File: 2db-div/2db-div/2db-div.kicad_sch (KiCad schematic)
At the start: 34 parts, among them J1001 Conn_01x02, J1002 From R2, J1003 Conn_01x02, J1004 Conn_Coaxial, SW1001 2dB, SW1002 Video, U1001 MC1458

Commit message: minor changes for spice
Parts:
- H1001, H1002, H1003, H1004, SW1002: Spice_Netlist_Enabled (none) -> N; Spice_Primitive (none) -> R
- J1002: Spice_Model (none) -> From R2; Spice_Netlist_Enabled (none) -> N; Spice_Primitive (none) -> J
- SW1001: Spice_Model (none) -> 2dB
- U1001: Spice_Lib_File 2db-div-spice\MC1458-dual.lib -> 2db-div-spice\LM358-dual.lib; Spice_Model MC1458_ti -> LM358c; Spice_Netlist_Enabled Y -> N
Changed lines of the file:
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@@
+      (effects (font (size 1.27 1.27)) hide)
+    )
+    (property "Spice_Primitive" "R" (id 4) (at 180.975 163.83 0)
+      (effects (font (size 1.27 1.27)) hide)
+    )
+    (property "Spice_Netlist_Enabled" "N" (id 5) (at 180.975 163.83 0)
       (effects (font (size 1.27 1.27)) hide)
     )
@@
       (effects (font (size 1.27 1.27)) hide)
     )
-    (property "Spice_Model" "MC1458_ti" (id 5) (at 132.08 82.55 0)
-      (effects (font (size 1.27 1.27)) hide)
-    )
-    (property "Spice_Netlist_Enabled" "Y" (id 6) (at 132.08 82.55 0)
-      (effects (font (size 1.27 1.27)) hide)
-    )
-    (property "Spice_Lib_File" "2db-div-spice\\MC1458-dual.lib" (id 7) (at 132.08 82.55 0)
+    (property "Spice_Model" "LM358c" (id 5) (at 132.08 82.55 0)
+      (effects (font (size 1.27 1.27)) hide)
+    )
+    (property "Spice_Netlist_Enabled" "N" (id 6) (at 132.08 82.55 0)
+      (effects (font (size 1.27 1.27)) hide)
+    )
+    (property "Spice_Lib_File" "2db-div-spice\\LM358-dual.lib" (id 7) (at 132.08 82.55 0)
       (effects (font (size 1.27 1.27)) hide)
     )
@@
       (effects (font (size 1.27 1.27)) hide)
     )
+    (property "Spice_Primitive" "R" (id 4) (at 227.33 85.09 0)
+      (effects (font (size 1.27 1.27)) hide)
+    )
+    (property "Spice_Netlist_Enabled" "N" (id 5) (at 227.33 85.09 0)
+      (effects (font (size 1.27 1.27)) hide)
+    )
     (pin "1")
     (pin "2")
@@
       (effects (font (size 1.27 1.27)) hide)
     )
+    (property "Spice_Primitive" "R" (id 4) (at 217.805 163.83 0)
+      (effects (font (size 1.27 1.27)) hide)
+    )
+    (property "Spice_Netlist_Enabled" "N" (id 5) (at 217.805 163.83 0)
+      (effects (font (size 1.27 1.27)) hide)
+    )
   )
   (symbol (lib_id "Mechanical:MountingHole") (at 163.195 163.83 0) (unit 1)
@@
     )
     (property "Datasheet" "~" (id 3) (at 163.195 163.83 0)
+      (effects (font (size 1.27 1.27)) hide)
+    )
+    (property "Spice_Primitive" "R" (id 4) (at 163.195 163.83 0)
+      (effects (font (size 1.27 1.27)) hide)
+    )
+    (property "Spice_Netlist_Enabled" "N" (id 5) (at 163.195 163.83 0)
       (effects (font (size 1.27 1.27)) hide)
     )
@@
     )
     (property "Datasheet" "~" (id 3) (at 198.755 163.83 0)
+      (effects (font (size 1.27 1.27)) hide)
+    )
+    (property "Spice_Primitive" "R" (id 4) (at 198.755 163.83 0)
+      (effects (font (size 1.27 1.27)) hide)
+    )
+    (property "Spice_Netlist_Enabled" "N" (id 5) (at 198.755 163.83 0)
       (effects (font (size 1.27 1.27)) hide)
     )
@@
       (effects (font (size 1.27 1.27)) hide)
     )
+    (property "Spice_Model" "2dB" (id 6) (at 208.28 77.47 0)
+      (effects (font (size 1.27 1.27)) hide)
+    )
     (pin "1")
     (pin "2")
@@
       (effects (font (size 1.27 1.27)) hide)
     )
-    (property "Spice_Model" "MC1458_ti" (id 5) (at 155.575 80.01 0)
-      (effects (font (size 1.27 1.27)) hide)
-    )
-    (property "Spice_Netlist_Enabled" "Y" (id 6) (at 155.575 80.01 0)
-      (effects (font (size 1.27 1.27)) hide)
-    )
-    (property "Spice_Lib_File" "2db-div-spice\\MC1458-dual.lib" (id 7) (at 155.575 80.01 0)
+    (property "Spice_Model" "LM358c" (id 5) (at 155.575 80.01 0)
+      (effects (font (size 1.27 1.27)) hide)
+    )
+    (property "Spice_Netlist_Enabled" "N" (id 6) (at 155.575 80.01 0)
+      (effects (font (size 1.27 1.27)) hide)
+    )
+    (property "Spice_Lib_File" "2db-div-spice\\LM358-dual.lib" (id 7) (at 155.575 80.01 0)
       (effects (font (size 1.27 1.27)) hide)
     )
@@
       (effects (font (size 1.27 1.27)) hide)
     )
-    (property "Spice_Model" "MC1458_ti" (id 5) (at 158.75 80.01 0)
-      (effects (font (size 1.27 1.27)) hide)
-    )
-    (property "Spice_Netlist_Enabled" "Y" (id 6) (at 158.75 80.01 0)
-      (effects (font (size 1.27 1.27)) hide)
-    )
-    (property "Spice_Lib_File" "2db-div-spice\\MC1458-dual.lib" (id 7) (at 158.75 80.01 0)
+    (property "Spice_Model" "LM358c" (id 5) (at 158.75 80.01 0)
+      (effects (font (size 1.27 1.27)) hide)
+    )
+    (property "Spice_Netlist_Enabled" "N" (id 6) (at 158.75 80.01 0)
+      (effects (font (size 1.27 1.27)) hide)
+    )
+    (property "Spice_Lib_File" "2db-div-spice\\LM358-dual.lib" (id 7) (at 158.75 80.01 0)
       (effects (font (size 1.27 1.27)) hide)
     )
@@
       (effects (font (size 1.27 1.27)) hide)
     )
+    (property "Spice_Primitive" "J" (id 4) (at 72.39 85.09 0)
+      (effects (font (size 1.27 1.27)) hide)
+    )
+    (property "Spice_Model" "From R2" (id 5) (at 72.39 85.09 0)
+      (effects (font (size 1.27 1.27)) hide)
+    )
+    (property "Spice_Netlist_Enabled" "N" (id 6) (at 72.39 85.09 0)
+      (effects (font (size 1.27 1.27)) hide)
+    )

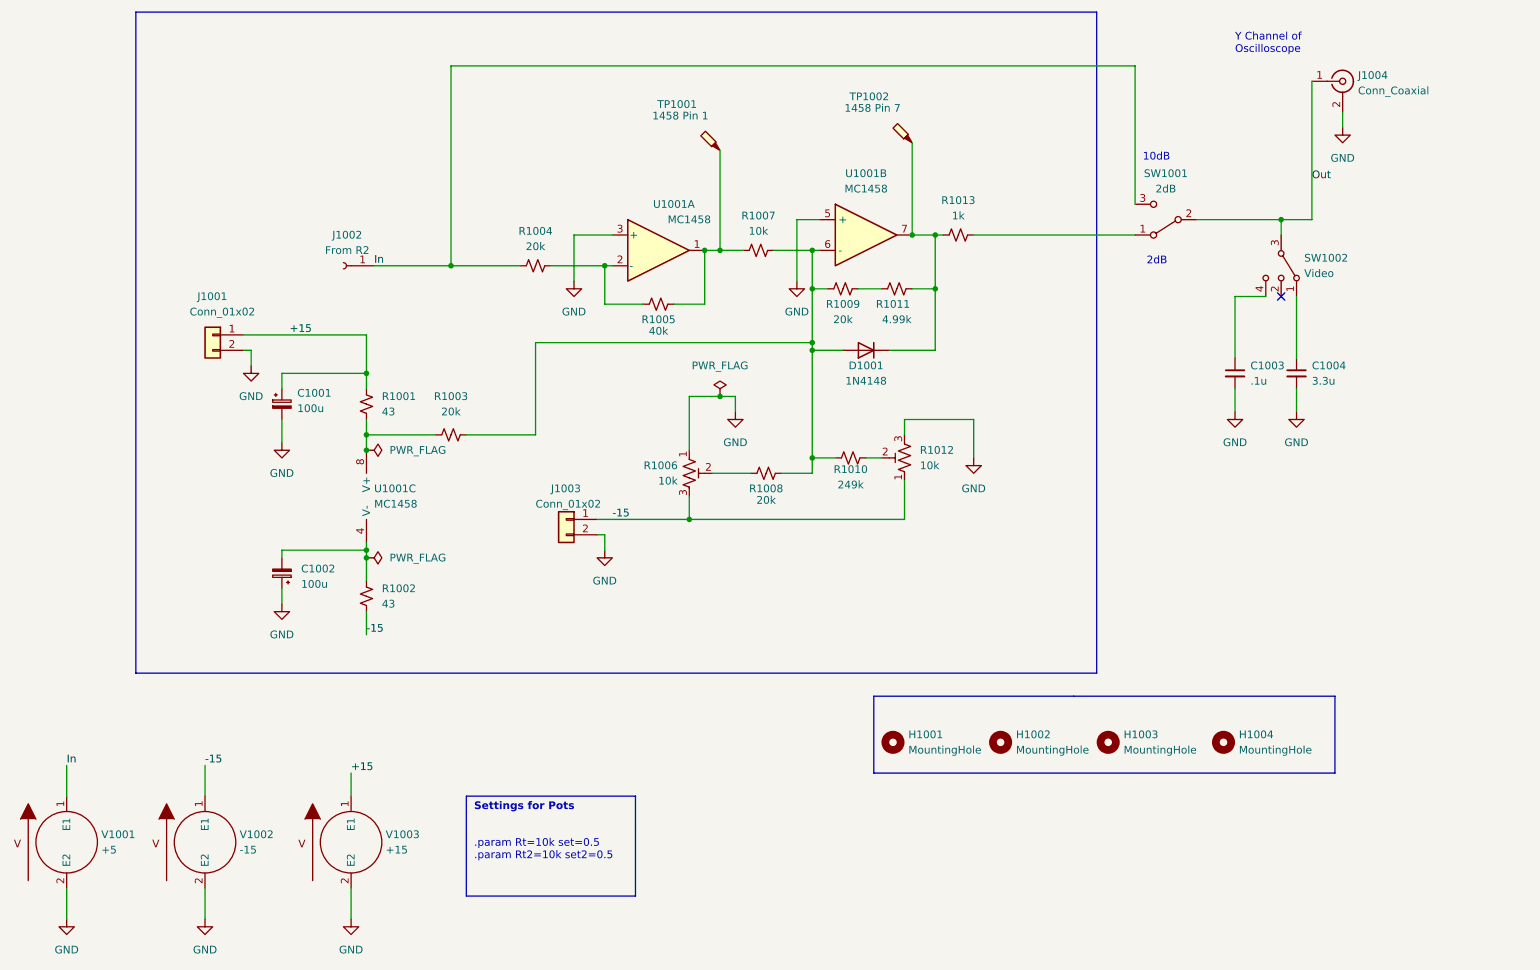
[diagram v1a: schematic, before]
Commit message: v7 conversion
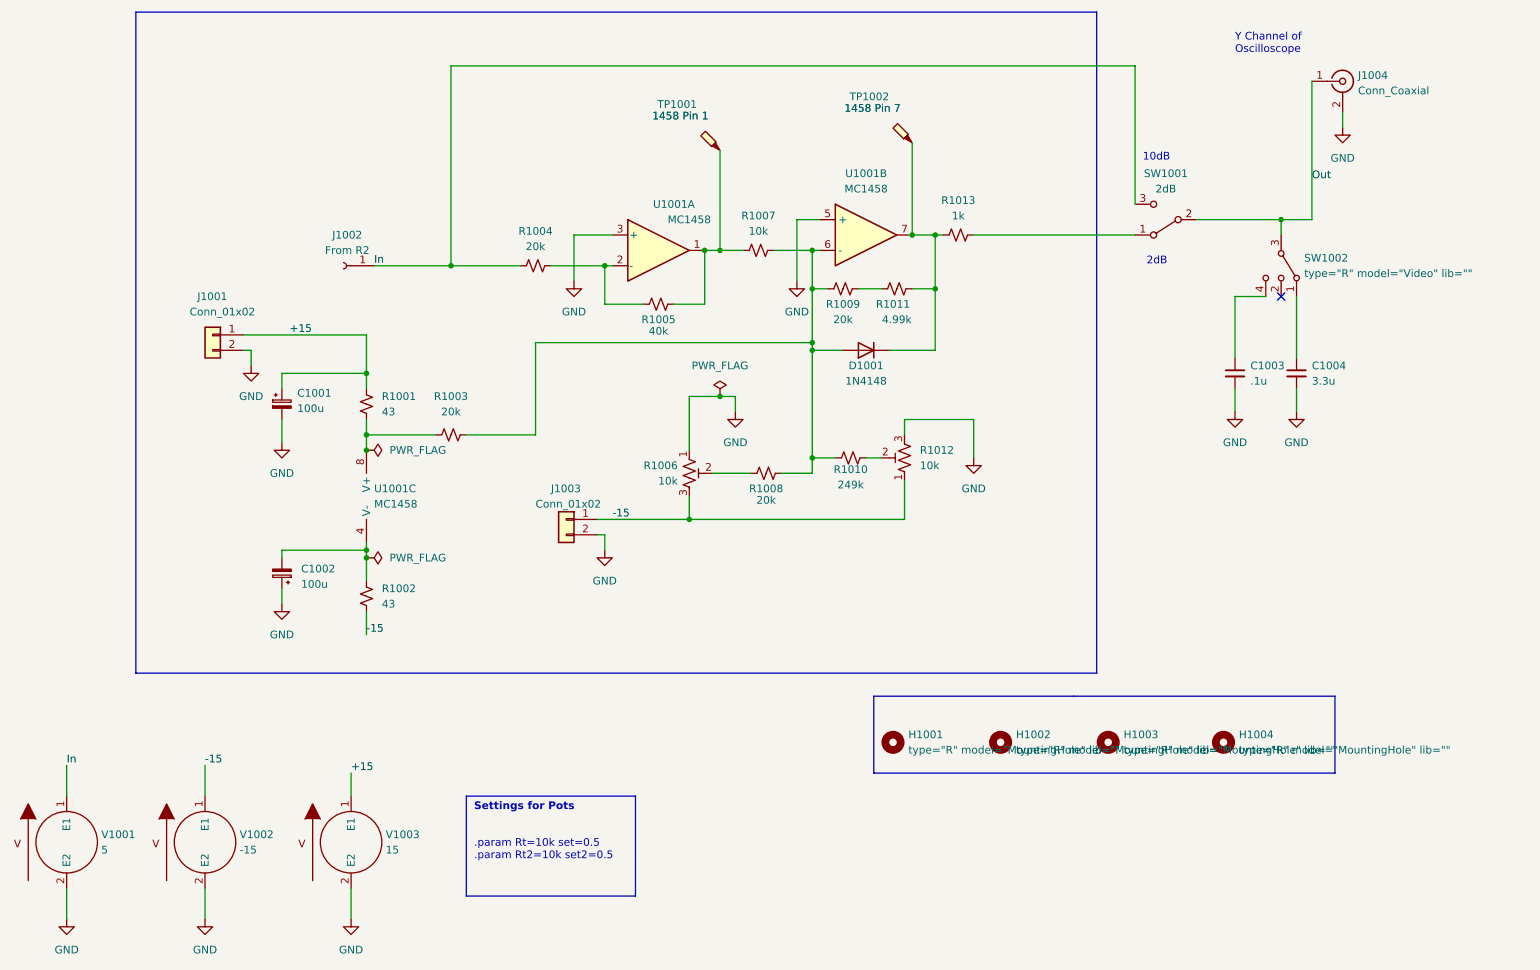
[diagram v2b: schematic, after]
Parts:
- D1001: Spice_Lib_File 2db-div-spice\fairch.lib -> (none); Spice_Model 1N4152 -> (none); Spice_Netlist_Enabled Y -> (none); Spice_Node_Sequence 2 1 -> (none); Spice_Primitive D -> (none)
- H1001, H1002, H1003, H1004: value MountingHole -> ${SIM.PARAMS}; Spice_Netlist_Enabled N -> (none); Spice_Primitive R -> (none)
- J1001, J1003: Spice_Model Conn_01x02 -> (none); Spice_Netlist_Enabled N -> (none); Spice_Primitive J -> (none)
- J1002: Spice_Model From R2 -> (none); Spice_Netlist_Enabled N -> (none); Spice_Primitive J -> (none)
- J1004: Spice_Model Conn_Coaxial -> (none); Spice_Netlist_Enabled N -> (none); Spice_Primitive J -> (none)
- R1006: Spice_Lib_File 2db-div-spice\Pot.lib -> (none); Spice_Model pot_lin -> (none); Spice_Netlist_Enabled Y -> (none); Spice_Primitive X -> (none)
- R1012: Spice_Lib_File 2db-div-spice\Pot2.lib -> (none); Spice_Model pot_lin2 -> (none); Spice_Netlist_Enabled Y -> (none); Spice_Primitive X -> (none)
- SW1001: Spice_Model 2dB -> (none); Spice_Netlist_Enabled N -> (none); Spice_Primitive R -> (none)
- SW1002: value Video -> ${SIM.PARAMS}; Spice_Netlist_Enabled N -> (none); Spice_Primitive R -> (none)
- TP1001: value 1458 Pin 1 -> ${SIM.PARAMS}; Spice_Netlist_Enabled N -> (none)
- TP1002: value 1458 Pin 7 -> ${SIM.PARAMS}; Spice_Netlist_Enabled N -> (none)
- U1001: Spice_Lib_File 2db-div-spice\LM358-dual.lib -> (none); Spice_Model LM358c -> (none); Spice_Netlist_Enabled N -> (none); Spice_Primitive X -> (none)
- V1001: value +5 -> 5; Spice_Model dc 5 -> (none); Spice_Netlist_Enabled Y -> (none); Spice_Primitive V -> (none)
- V1002: Spice_Model dc -15 -> (none); Spice_Netlist_Enabled Y -> (none); Spice_Primitive V -> (none)
- V1003: value +15 -> 15; Spice_Model dc 15 -> (none); Spice_Netlist_Enabled Y -> (none); Spice_Primitive V -> (none)
